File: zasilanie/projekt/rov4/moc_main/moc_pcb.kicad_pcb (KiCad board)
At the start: 2 copper layers, 296.5 x 109.2 mm, 88 parts, among them IC2 UWE-12_10-Q12PB-C, J27 High power: ON-OFF, J28 ESC1, J29 ESC2, J30 ESC3, J31 ESC4, J32 ESC5, J33 ESC6, J34 ESC7, J35 ESC8, J36 Extra, J37 Torp_EleMagnes, J38 Extra, J39 RC: 12V, J40 Manip_Silnik_3, J41 Manip_Silnik_1, J42 Manip_Silnik_2, J52 HP_OUT, J58 +BattPower, J59 -BattPower, J62 bus_bar, J63 bus_bar, J64 bus_bar, J65 bus_bar, J66 bus_bar, J67 bus_bar, J68 bus_bar_bott, J69 bus_bar_bott, J70 bus_bar_bott, J71 bus_bar_bott, J72 bus_bar_bott, J73 bus_bar_bott, J74 bus_bar_bott, J75 bus_bar_bott, J76 bus_bar_bott, J77 bus_bar_bott, J78 bus_bar_bott, J80 BatPow_Sens, Q6 IPT004N03L, Q7 IPT004N03L, Q8 IPT004N03L, Q9 IPT004N03L, U2 Transoptor, U3 Transoptor

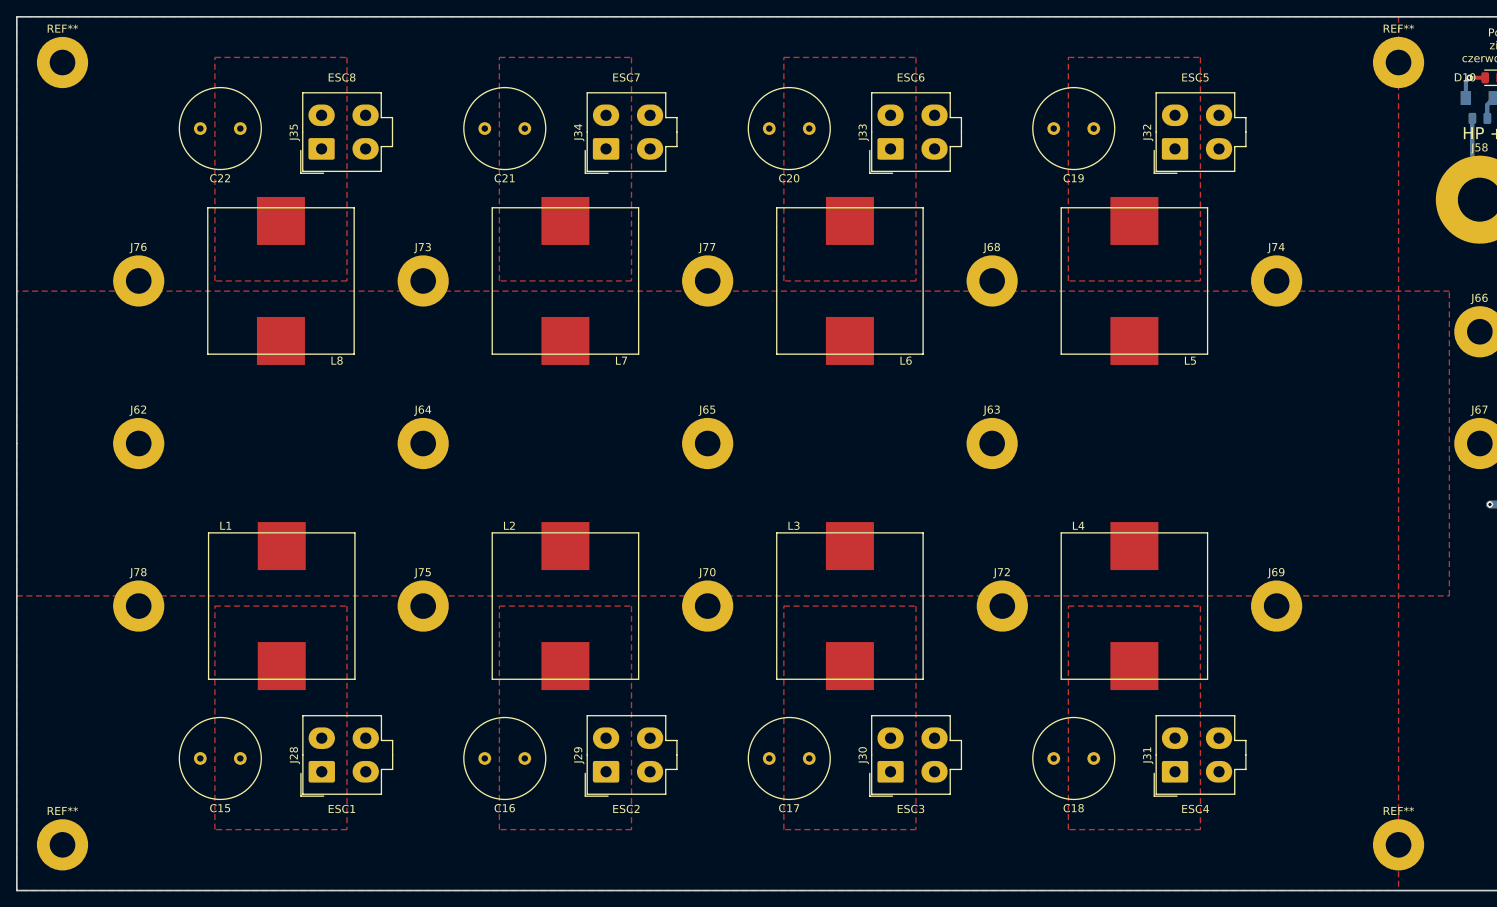
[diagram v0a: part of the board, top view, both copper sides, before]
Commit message: kosmetyka
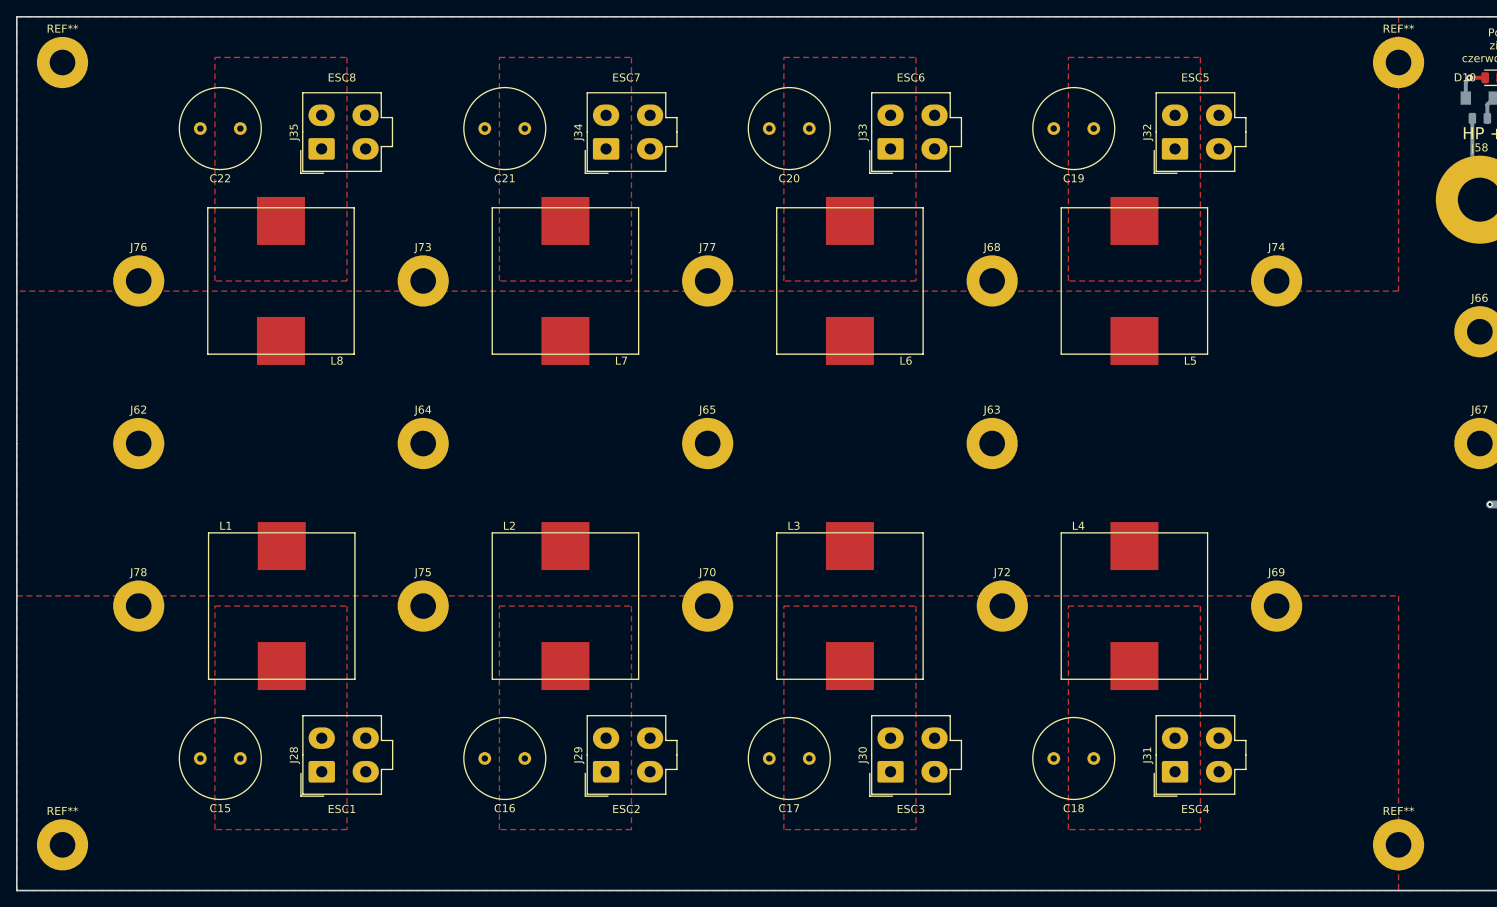
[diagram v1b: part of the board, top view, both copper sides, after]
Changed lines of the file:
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@@
     (46 B.CrtYd user)
     (47 F.CrtYd user)
-    (48 B.Fab user hide)
+    (48 B.Fab user)
     (49 F.Fab user)
   )
@@
       (rotate (xyz 0 0 0))
     )
+    (model C:/Users/Kurat/Documents/git_repos/Rov4/zasilanie/modele_3d/C_Radial_D10.0mm_H20.0mm_P5.00mm.stp
+      (offset (xyz 2.5 0 0))
+      (scale (xyz 1 1 1))
+      (rotate (xyz -90 0 90))
+    )
   )
   (module Capacitor_THT:C_Radial_D10.0mm_H20.0mm_P5.00mm (layer F.Cu)
@@
       (rotate (xyz 0 0 0))
     )
+    (model C:/Users/Kurat/Documents/git_repos/Rov4/zasilanie/modele_3d/C_Radial_D10.0mm_H20.0mm_P5.00mm.stp
+      (offset (xyz 2.5 0 0))
+      (scale (xyz 1 1 1))
+      (rotate (xyz -90 0 90))
+    )
   )
   (module Capacitor_THT:C_Radial_D10.0mm_H20.0mm_P5.00mm (layer F.Cu)
@@
       (rotate (xyz 0 0 0))
     )
+    (model C:/Users/Kurat/Documents/git_repos/Rov4/zasilanie/modele_3d/C_Radial_D10.0mm_H20.0mm_P5.00mm.stp
+      (offset (xyz 2.5 0 0))
+      (scale (xyz 1 1 1))
+      (rotate (xyz -90 0 90))
+    )
   )
   (module Capacitor_THT:C_Radial_D10.0mm_H20.0mm_P5.00mm (layer F.Cu)
@@
       (net 5 "Net-(C18-Pad1)"))
     (model ${KISYS3DMOD}/Capacitor_THT.3dshapes/C_Radial_D10.0mm_H20.0mm_P5.00mm.wrl
-      (at (xyz 0 0 0))
+      (offset (xyz 2.5 0 0))
       (scale (xyz 1 1 1))
-      (rotate (xyz 0 0 0))
+      (rotate (xyz -90 0 90))
+    )
+    (model C:/Users/Kurat/Documents/git_repos/Rov4/zasilanie/modele_3d/C_Radial_D10.0mm_H20.0mm_P5.00mm.stp
+      (offset (xyz 2.5 0 0))
+      (scale (xyz 1 1 1))
+      (rotate (xyz -90 0 90))
     )
   )
@@
       (rotate (xyz 0 0 0))
     )
+    (model C:/Users/Kurat/Documents/git_repos/Rov4/zasilanie/modele_3d/C_Radial_D10.0mm_H20.0mm_P5.00mm.stp
+      (offset (xyz 2.5 0 0))
+      (scale (xyz 1 1 1))
+      (rotate (xyz -90 0 90))
+    )
   )
   (module Capacitor_THT:C_Radial_D10.0mm_H20.0mm_P5.00mm (layer F.Cu)
@@
       (rotate (xyz 0 0 0))
     )
+    (model C:/Users/Kurat/Documents/git_repos/Rov4/zasilanie/modele_3d/C_Radial_D10.0mm_H20.0mm_P5.00mm.stp
+      (offset (xyz 2.5 0 0))
+      (scale (xyz 1 1 1))
+      (rotate (xyz -90 0 90))
+    )
   )
   (module Capacitor_THT:C_Radial_D10.0mm_H20.0mm_P5.00mm (layer F.Cu)
@@
       (rotate (xyz 0 0 0))
     )
+    (model C:/Users/Kurat/Documents/git_repos/Rov4/zasilanie/modele_3d/C_Radial_D10.0mm_H20.0mm_P5.00mm.stp
+      (offset (xyz 2.5 0 0))
+      (scale (xyz 1 1 1))
+      (rotate (xyz -90 0 90))
+    )
   )
   (module Capacitor_SMD:CP_Elec_6.3x5.4 (layer B.Cu)
@@
       (rotate (xyz 0 0 0))
     )
+    (model C:/Users/Kurat/Documents/git_repos/Rov4/zasilanie/modele_3d/spox_2pin_socket_pcb.stp
+      (offset (xyz 1.25 0.63 1.5))
+      (scale (xyz 1 1 1))
+      (rotate (xyz -90 0 180))
+    )
   )
   (module Connector_Molex:Molex_Mini-Fit_Jr_5566-04A_2x02_P4.20mm_Vertical (layer F.Cu)
@@
       (rotate (xyz 0 0 0))
     )
+    (model C:/Users/Kurat/Documents/git_repos/Rov4/zasilanie/modele_3d/spox_2pin_socket_pcb.stp
+      (offset (xyz 1.25 0.63 1.5))
+      (scale (xyz 1 1 1))
+      (rotate (xyz -90 0 180))
+    )
   )
   (module Connector_Molex:Molex_Mini-Fit_Jr_5566-04A_2x02_P4.20mm_Vertical (layer F.Cu)
@@
       (rotate (xyz 0 0 0))
     )
+    (model "C:/Users/Kurat/Documents/git_repos/Rov4/zasilanie/modele_3d/molex 2x2 socket pcb.stp"
+      (offset (xyz 2.1 -2.5 0))
+      (scale (xyz 1 1 1))
+      (rotate (xyz -90 0 180))
+    )
   )
   (module 74435571100:74435571100 (layer F.Cu)
@@
       (rotate (xyz 0 0 0))
     )
+    (model C:/Users/Kurat/Documents/git_repos/Rov4/zasilanie/modele_3d/spox_2pin_socket_pcb.stp
+      (offset (xyz 1.25 0.63 1.5))
+      (scale (xyz 1 1 1))
+      (rotate (xyz -90 0 180))
+    )
   )
   (gr_text "Polaryzacja: \nzielone - ok\nczerwone - odwrotnie" (at 202.752 18.332) (layer F.SilkS)
@@
     (polygon
       (pts
-        (xy 191.262 49.022) (xy 193.802 46.482) (xy 201.422 46.482) (xy 203.962 49.022) (xy 203.962 69.342)
-        (xy 202.692 71.882) (xy 201.422 73.152) (xy 198.882 74.422) (xy 24.892 74.422) (xy 22.352 71.882)
-        (xy 22.352 64.262) (xy 24.892 61.722) (xy 191.262 61.722)
+        (xy 191.262 49.022) (xy 193.802 46.482) (xy 201.422 46.482) (xy 203.962 49.022) (xy 203.962 71.882)
+        (xy 201.422 74.422) (xy 24.892 74.422) (xy 22.352 71.882) (xy 22.352 64.262) (xy 24.892 61.722)
+        (xy 191.262 61.722)
       )
     )
@@
     (polygon
       (pts
-        (xy 231.902 84.582) (xy 229.362 82.042) (xy 178.562 82.042) (xy 178.562 46.482) (xy 177.292 43.942)
-        (xy 176.022 42.672) (xy 173.482 41.402) (xy 26.162 41.402) (xy 22.352 43.942) (xy 22.352 51.562)
-        (xy 24.892 54.102) (xy 165.862 54.102) (xy 165.862 82.042) (xy 24.892 82.042) (xy 22.352 84.582)
-        (xy 22.352 92.202) (xy 24.892 94.742) (xy 229.362 94.742) (xy 231.902 92.202)
-      )
-    )
-  )
-  (zone (net 10) (net_name +BattPow) (layer F.Cu) (hatch edge 0.508)
-    (connect_pads (clearance 0.4))
-    (min_thickness 0.254)
-    (fill yes (arc_segments 32) (thermal_gap 0.508) (thermal_bridge_width 3) (smoothing chamfer) (radius 3))
-    (polygon
-      (pts
-        (xy 193.802 49.022) (xy 14.732 49.022) (xy 14.732 87.122) (xy 193.802 87.122)
+        (xy 231.902 84.582) (xy 229.362 82.042) (xy 178.562 82.042) (xy 178.562 44.196) (xy 176.022 41.656)
+        (xy 24.892 41.402) (xy 22.352 43.942) (xy 22.352 51.562) (xy 24.892 54.102) (xy 165.862 54.102)
+        (xy 165.862 82.042) (xy 24.892 82.042) (xy 22.352 84.582) (xy 22.352 92.202) (xy 24.892 94.742)
+        (xy 229.362 94.742) (xy 231.902 92.202)
       )
     )
@@
     (polygon
       (pts
-        (xy 187.452 14.732) (xy 187.452 123.952) (xy 254.762 123.952) (xy 254.762 84.582) (xy 240.157 69.977)
-        (xy 240.157 52.197) (xy 260.477 31.877) (xy 260.477 14.732)
+        (xy 187.452 14.732) (xy 187.452 49.022) (xy 14.732 49.022) (xy 14.732 87.122) (xy 187.452 87.122)
+        (xy 187.452 123.952) (xy 254.762 123.952) (xy 254.762 84.582) (xy 240.157 69.977) (xy 240.157 52.197)
+        (xy 260.477 31.877) (xy 260.477 14.732)
       )
     )
